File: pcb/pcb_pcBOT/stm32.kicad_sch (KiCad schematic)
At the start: 0 parts

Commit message: fin bms schematic bms
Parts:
- added U303: STM32G431KBT6, Package_QFP:LQFP-32_7x7mm_P0.8mm, symbol MCU_ST_STM32G4:STM32G431KBTx
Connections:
- new net: U303.16 (VSS), U303.32 (VSS)
- new net I2C_SCL: U303.31 (PB8)
- new net I2C_SDA: U303.30 (PB7)
- new net MOT_AIN1: U303.18 (PA8)
- new net MOT_AIN2: U303.21 (PA11)
- new net MOT_BIN1: U303.19 (PA9)
- new net MOT_BIN2: U303.22 (PA12)
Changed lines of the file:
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@@
 	(generator_version "9.0")
 	(paper "A4")
+	(hierarchical_label "MOT_BIN2"
+		(shape bidirectional)
+		(at 105.41 86.36 0)
+		(effects
+			(font
+				(size 1.27 1.27)
+			)
+			(justify left)
+		)
+	)
+	(hierarchical_label "MOT_AIN2"
+		(shape bidirectional)
+		(at 105.41 83.82 0)
+		(effects
+			(font
+				(size 1.27 1.27)
+			)
+			(justify left)
+		)
+	)
+	(hierarchical_label "I2C_SCL"
+		(shape bidirectional)
+		(at 80.01 83.82 180)
+		(effects
+			(font
+				(size 1.27 1.27)
+			)
+			(justify right)
+		)
+	)
+	(hierarchical_label "MOT_AIN1"
+		(shape bidirectional)
+		(at 105.41 76.2 0)
+		(effects
+			(font
+				(size 1.27 1.27)
+			)
+			(justify left)
+		)
+	)
+	(hierarchical_label "I2C_SDA"
+		(shape bidirectional)
+		(at 80.01 81.28 180)
+		(effects
+			(font
+				(size 1.27 1.27)
+			)
+			(justify right)
+		)
+	)
+	(hierarchical_label "MOT_BIN1"
+		(shape bidirectional)
+		(at 105.41 78.74 0)
+		(effects
+			(font
+				(size 1.27 1.27)
+			)
+			(justify left)
+		)
+	)
+	(symbol
+		(lib_id "MCU_ST_STM32G4:STM32G431KBTx")
+		(at 92.71 76.2 0)
+		(unit 1)
+		(exclude_from_sim no)
+		(in_bom yes)
+		(on_board yes)
+		(dnp no)
+		(fields_autoplaced yes)
+		(property "Reference" "U303"
+			(at 97.3933 101.6 0)
+			(effects
+				(font
+					(size 1.27 1.27)
+				)
+				(justify left)
+			)
+		)
+		(property "Value" "STM32G431KBT6"
+			(at 97.3933 104.14 0)
+			(effects
+				(font
+					(size 1.27 1.27)
+				)
+				(justify left)
+			)
+		)
+		(property "Footprint" "Package_QFP:LQFP-32_7x7mm_P0.8mm"
+			(at 82.55 99.06 0)
+			(effects
+				(font
+					(size 1.27 1.27)
+				)
+				(justify right)
+				(hide yes)
+			)
+		)
+		(property "Datasheet" "https://www.st.com/resource/en/datasheet/stm32g431kb.pdf"
+			(at 92.71 76.2 0)
+			(effects
+				(font
+					(size 1.27 1.27)
+				)
+				(hide yes)
+			)
+		)
+		(property "Description" "STMicroelectronics Arm Cortex-M4 MCU, 128KB flash, 32KB RAM, 170 MHz, 1.71-3.6V, 26 GPIO, LQFP32"
+			(at 92.71 76.2 0)
+			(effects
+				(font
+					(size 1.27 1.27)
+				)
+				(hide yes)
+			)
+		)
+		(pin "16"
+		)
+		(pin "5"
+		)
+		(pin "13"
+		)
+		(pin "28"
+		)
+		(pin "29"
+		)
+		(pin "27"
+		)
+		(pin "31"
+		)
+		(pin "4"
+		)
+		(pin "3"
+		)
+		(pin "1"
+		)
+		(pin "17"
+		)
+		(pin "15"
+		)
+		(pin "14"
+		)
+		(pin "2"
+		)
+		(pin "26"
+		)
+		(pin "30"
+		)
+		(pin "32"
+		)
+		(pin "22"
+		)
+		(pin "9"
+		)
+		(pin "11"
+		)
+		(pin "6"
+		)
+		(pin "21"
+		)
+		(pin "18"
+		)
+		(pin "24"
+		)
+		(pin "7"
+		)
+		(pin "10"
+		)
+		(pin "12"
+		)
+		(pin "19"
+		)
+		(pin "8"
+		)
+		(pin "23"
+		)
+		(pin "20"
+		)
+		(pin "25"
+		)
+		(instances
+			(project ""
+				(path "/704e4da3-8ee7-458f-8a0f-3fc97e8dc2a6/d5d6119d-1191-46c1-ad63-61bb867f116c"
+					(reference "U303")
+					(unit 1)
+				)
+			)
+		)
+	)
 )

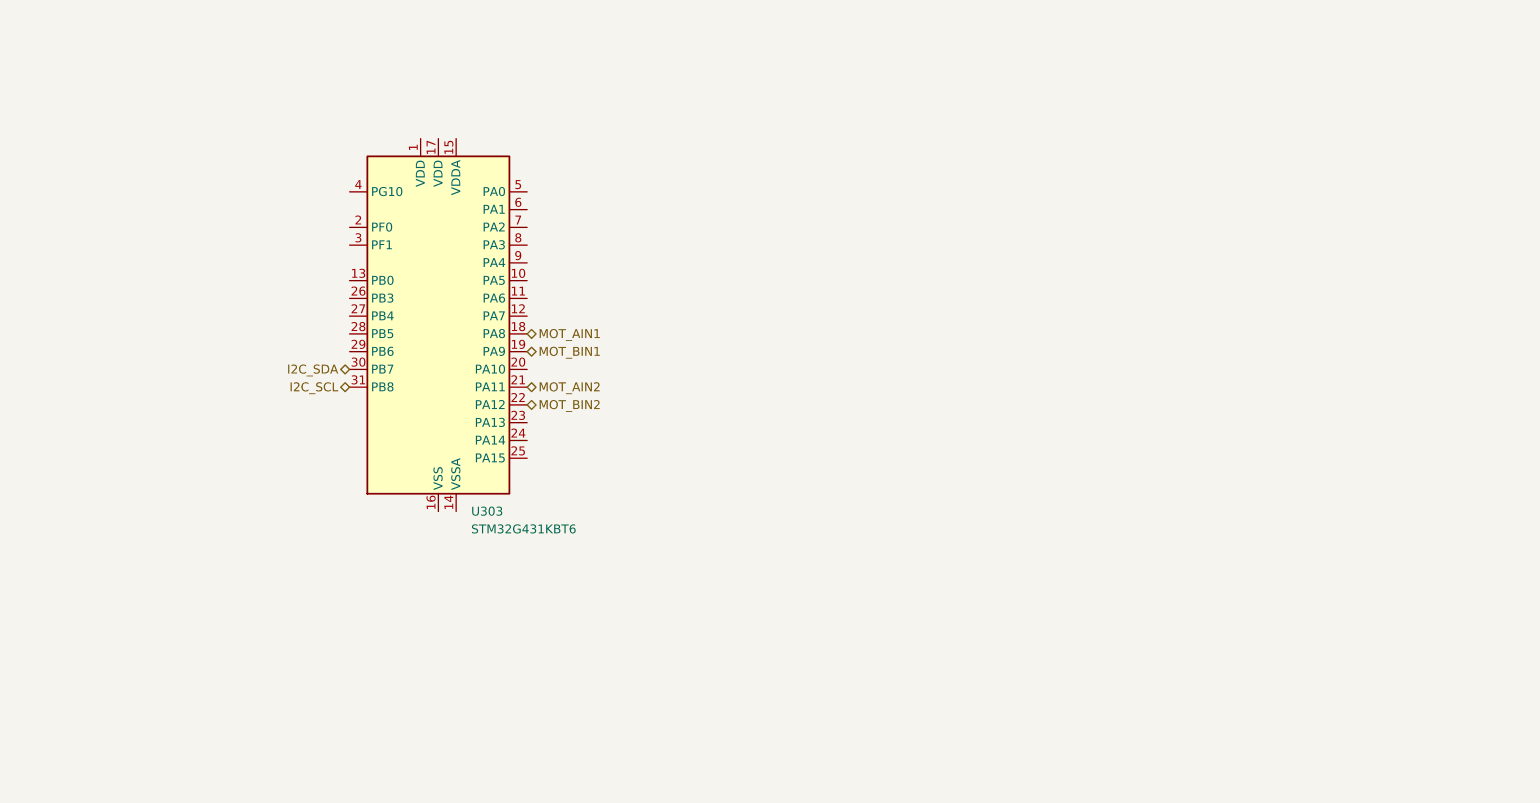
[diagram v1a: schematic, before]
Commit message: stm32 (in progress)
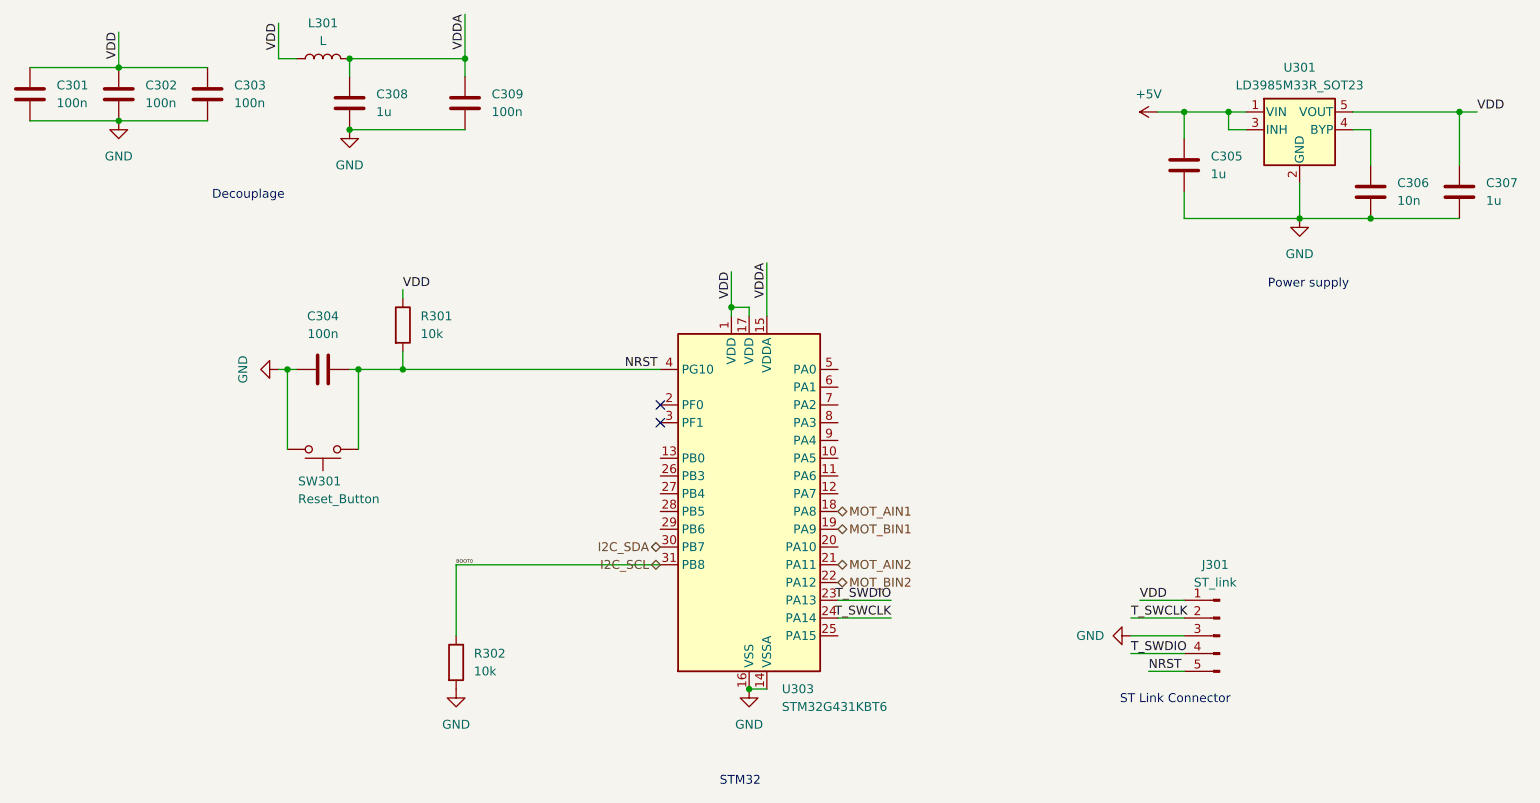
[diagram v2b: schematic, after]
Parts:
- added C301, C302, C303, C304, C309: 100n, symbol Device:C
- added C305, C307, C308: 1u, symbol Device:C
- added C306: 10n, symbol Device:C
- added J301: ST_link, symbol Connector:Conn_01x05_Pin
- added L301: L, symbol Device:L
- added R301, R302: 10k, symbol Device:R
- added SW301: Reset_Button, symbol Switch:SW_Push
- added U301: LD3985M33R_SOT23, Package_TO_SOT_SMD:SOT-23-5, symbol Regulator_Linear:LD3985M33R_SOT23
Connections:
- net I2C_SCL: now also R302.1
- net VDD: now reaches U303.1 (VDD)
- net VDD: now also U303.17 (VDD), C301.1, C302.1, C303.1, C307.1, J301.1 (Pin_1), L301.1, R301.1, U301.5 (VOUT)
- net GND: now reaches U303.14 (VSSA)
- net GND: now also U303.16 (VSS), U303.32 (VSS), C301.2, C302.2, C303.2, C304.2, C305.2, C306.2, C307.2, C308.2, C309.2, J301.3 (Pin_3), R302.2, SW301.2, U301.2 (GND)
- net VDDA: now reaches U303.15 (VDDA)
- net VDDA: now also C308.1, C309.1, L301.2
- net T_SWDIO: now reaches U303.23 (PA13)
- net T_SWDIO: now also J301.4 (Pin_4)
- net T_SWCLK: now reaches U303.24 (PA14)
- net T_SWCLK: now also J301.2 (Pin_2)
- net NRST: now reaches U303.4 (PG10)
- net NRST: now also C304.1, J301.5 (Pin_5), R301.2, SW301.1
- new net: C306.1, U301.4 (BYP)
- new net +5V: C305.1, U301.1 (VIN), U301.3 (INH)
- no-connect marks 0 -> 2
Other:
- note added: "Decouplage"
- note added: "Power supply"
- note added: "ST Link Connector"
- note added: "STM32"
- moved on the sheet: U303
